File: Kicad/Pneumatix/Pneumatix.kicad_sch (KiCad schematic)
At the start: 16 parts, among them J1 436500404, J2 142-0701-801, J3 Conn_01x04_Socket, U1 E22-400T33S

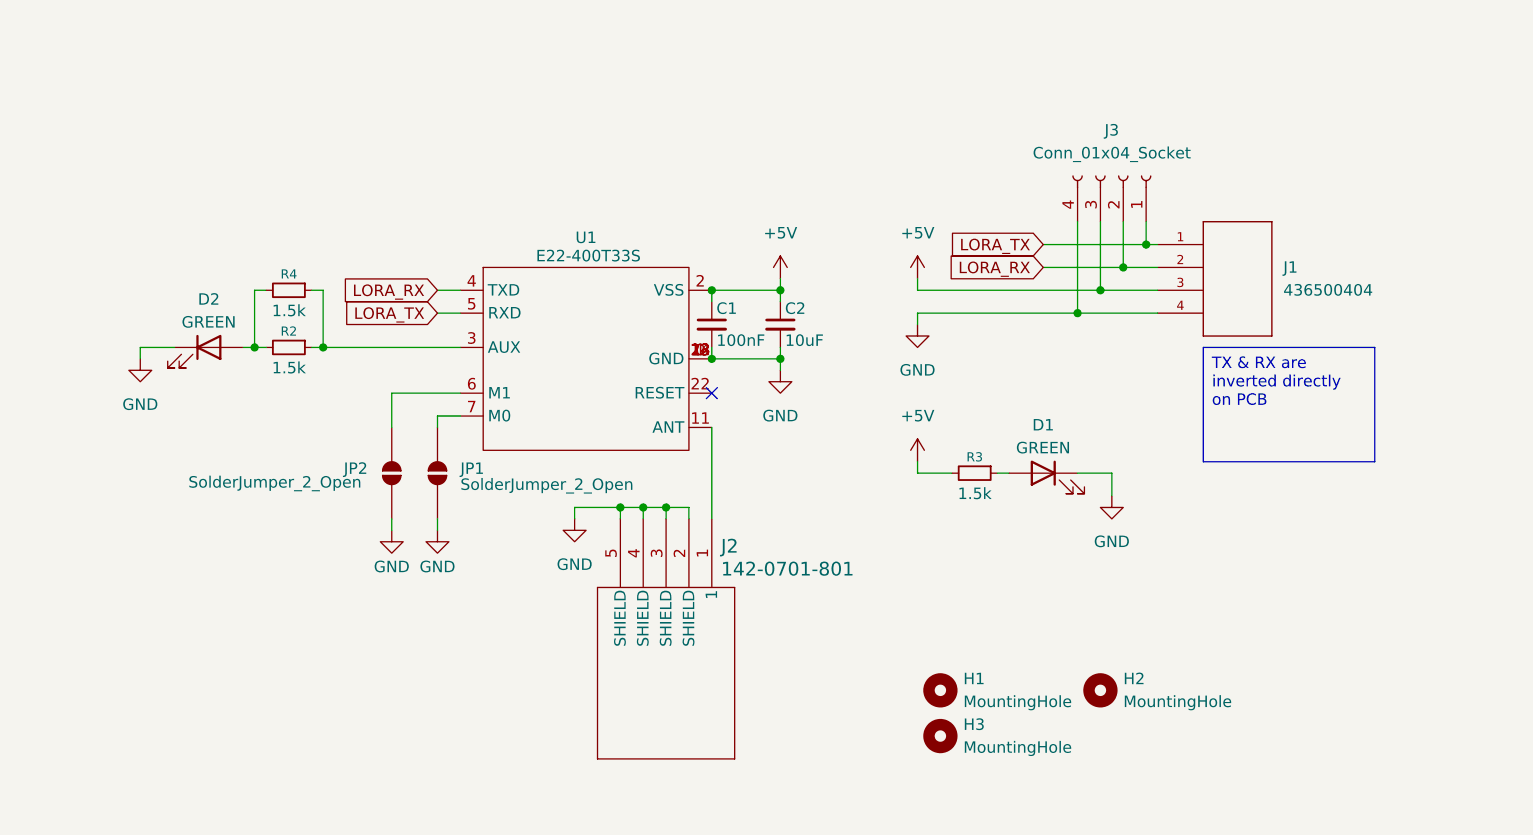
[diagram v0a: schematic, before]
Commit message: wip: add pu/pd for M0 and M1, remake traces and swap gnd/signal/passive components plane
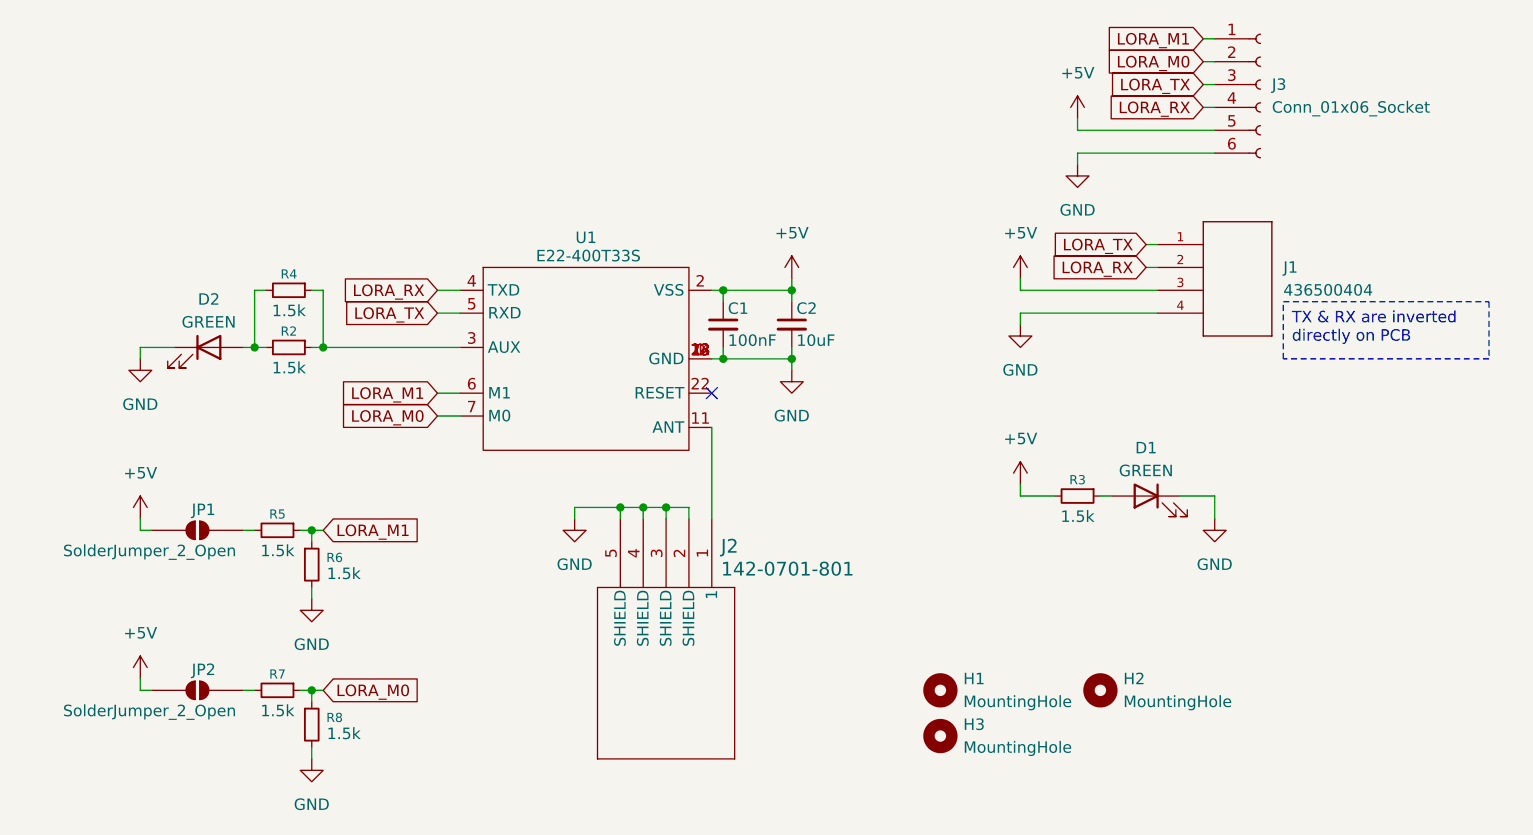
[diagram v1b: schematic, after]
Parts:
- removed J3: Conn_01x04_Socket, Connector_PinSocket_2.54mm:PinSocket_1x04_P2.54mm_Vertical, symbol Connector:Conn_01x04_Socket
- added J3: Conn_01x06_Socket, Connector_PinHeader_2.54mm:PinHeader_1x06_P2.54mm_Vertical, symbol Connector:Conn_01x06_Socket
- added R5, R6, R7, R8: 1.5k, Resistor_SMD:R_0603_1608Metric, symbol Device:R_Small
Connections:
- net +5V: now also JP1.2 (B), JP2.2 (B), J3.5 (Pin_5)
- net GND: now also J3.6 (Pin_6), R6.2, R8.2; no longer JP1.2 (B), JP2.2 (B)
- net LORA_RX: now also J3.4 (Pin_4)
- net LORA_TX: now also J3.3 (Pin_3)
- net at JP1.1 (A): now also R5.2; no longer U1.7 (M0)
- net at JP2.1 (A): now also R7.2; no longer U1.6 (M1)
- new net LORA_M0: J3.2 (Pin_2), R7.1, R8.1, U1.7 (M0)
- new net LORA_M1: J3.1 (Pin_1), R5.1, R6.1, U1.6 (M1)
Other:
- moved on the sheet: C1, C2, D1, JP1, R3
